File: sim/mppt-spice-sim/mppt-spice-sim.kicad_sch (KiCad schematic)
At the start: 8 parts, among them M1 mnmos1

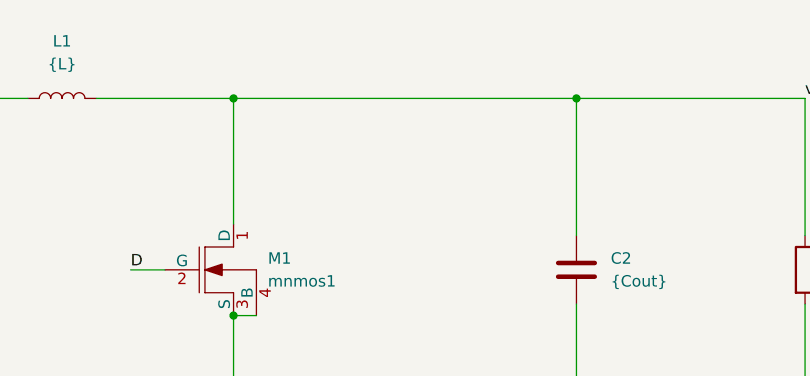
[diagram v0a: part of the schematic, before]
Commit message: commit last run of sw
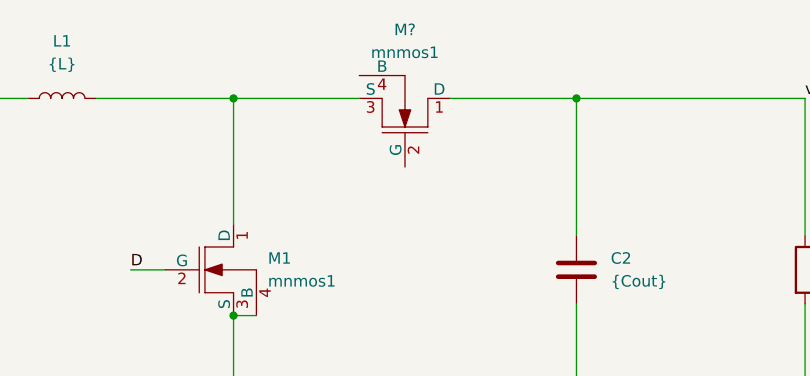
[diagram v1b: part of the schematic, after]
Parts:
- added M?: mnmos1, symbol pspice:MNMOS
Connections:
- net v_out: now also M?.1 (D); no longer L1.2, M1.1 (D)
- new net: L1.2, M1.1 (D), M?.3 (S)
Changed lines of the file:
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@@
+    (stroke (width 0) (type default) (color 0 0 0 0))
+  )
+  (wire (pts (xy 95.25 38.1) (xy 109.22 38.1))
     (stroke (width 0) (type default) (color 0 0 0 0))
   )
@@
     (stroke (width 0) (type default) (color 0 0 0 0))
   )
-  (wire (pts (xy 95.25 38.1) (xy 133.35 38.1))
-    (stroke (width 0) (type default) (color 0 0 0 0))
-  )
   (wire (pts (xy 133.35 38.1) (xy 158.75 38.1))
     (stroke (width 0) (type default) (color 0 0 0 0))
@@
   )
   (wire (pts (xy 38.1 76.2) (xy 57.15 76.2))
+    (stroke (width 0) (type default) (color 0 0 0 0))
+  )
+  (wire (pts (xy 119.38 38.1) (xy 133.35 38.1))
     (stroke (width 0) (type default) (color 0 0 0 0))
   )
@@
     (pin "2")
   )
+  (symbol (lib_id "pspice:MNMOS") (at 114.3 40.64 270) (mirror x) (unit 1)
+    (in_bom yes) (on_board yes) (fields_autoplaced)
+    (property "Reference" "M?" (id 0) (at 114.3 30.48 90))
+    (property "Value" "mnmos1" (id 1) (at 114.3 33.02 90))
+    (property "Footprint" "" (id 2) (at 114.3 41.275 0)
+      (effects (font (size 1.27 1.27)) hide)
+    )
+    (property "Datasheet" "~" (id 3) (at 114.3 41.275 0)
+      (effects (font (size 1.27 1.27)) hide)
+    )
+    (pin "1")
+    (pin "2")
+    (pin "3")
+    (pin "4")
+  )
   (sheet_instances
     (path "/" (page "1"))
@@
       (reference "M1") (unit 1) (value "mnmos1") (footprint "")
     )
+    (path "/fde5b2d6-1cb8-4f53-aa1f-0afb05f35974"
+      (reference "M?") (unit 1) (value "mnmos1") (footprint "")
+    )
     (path "/9e0c91bc-3a86-452b-8228-261d0cc52d68"
